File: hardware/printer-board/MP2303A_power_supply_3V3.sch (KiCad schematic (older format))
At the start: 10 parts, among them U12 MP2303A_ALT

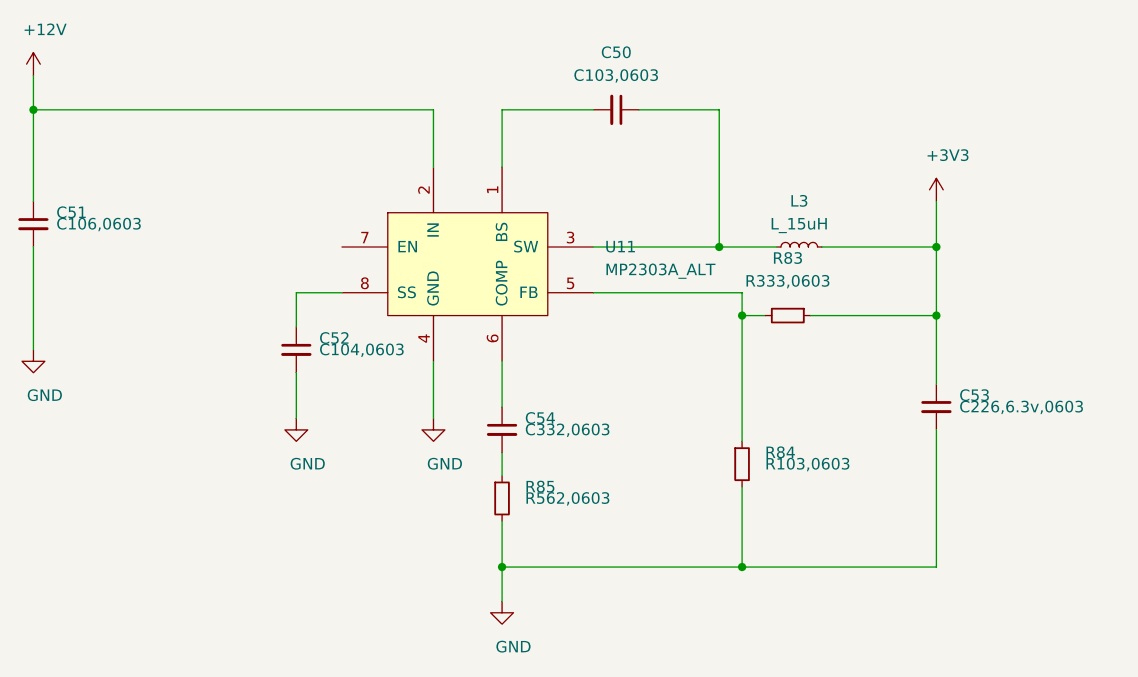
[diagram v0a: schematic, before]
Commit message: update to re-annotation,
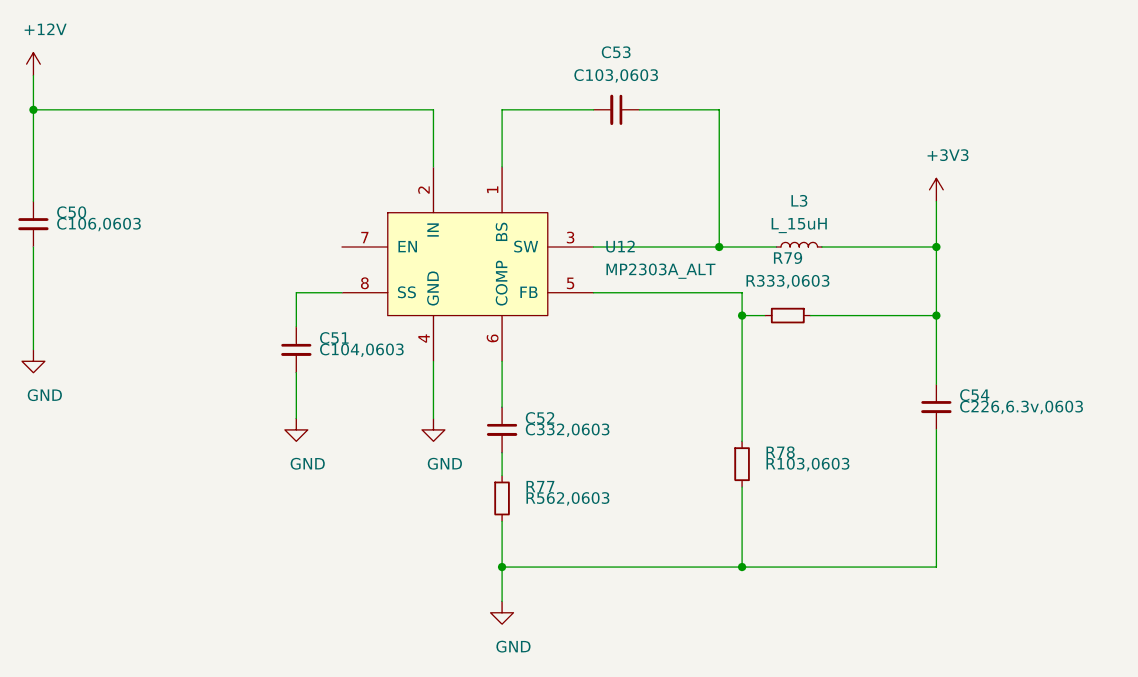
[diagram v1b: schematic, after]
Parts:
- U12: footprint Package_SO:SOIC-8_3.9x4.9mm_P1.27mm -> footprint-lib:SOIC-8_3.9x4.9mm_P1.27mm,thermal_via
- renumbered C54 to C52, C49 to C53, C53 to C54, L4 to L3, R91 to R77, R90 to R78, R89 to R79
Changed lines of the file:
@@
 $Descr A4 11693 8268
 encoding utf-8
-Sheet 34 29
+Sheet 29 29
 Title ""
 Date ""
@@
 $EndBitmap
 $Comp
-L taobao-components:MP2303A_ALT U12
+L taobao-components:MP2303A_ALT U?
 U 1 1 5CCACF42
 P 5000 3500
-AR Path="/5CC86276/5CCACF42" Ref="U12"  Part="1"
+AR Path="/5CC86276/5CCACF42" Ref="U?"  Part="1"
 AR Path="/5CCA7EF8/5CCACF42" Ref="U?"  Part="1"
 AR Path="/5CC29851/5CCA8098/5CCACF42" Ref="U?"  Part="1"
-AR Path="/5CCA8A04/5CCACF42" Ref="U11"  Part="1"
-F 0 "U11" H 5600 3550 50  0000 L CNN
+AR Path="/5CCA8A04/5CCACF42" Ref="U12"  Part="1"
+F 0 "U12" H 5600 3550 50  0000 L CNN
 F 1 "MP2303A_ALT" H 5600 3450 50  0000 L CNN
-F 2 "Package_SO:SOIC-8_3.9x4.9mm_P1.27mm" H 5000 3500 50  0001 C CNN
+F 2 "footprint-lib:SOIC-8_3.9x4.9mm_P1.27mm,thermal_via" H 5000 3500 50  0001 C CNN
 F 3 "" H 5000 3500 50  0001 C CNN
 	1    5000 3500
@@
 $EndComp
 $Comp
-L power:+12V #PWR0131
+L power:+12V #PWR?
 U 1 1 5CCACF43
 P 3100 2700
-AR Path="/5CC86276/5CCACF43" Ref="#PWR0131"  Part="1"
+AR Path="/5CC86276/5CCACF43" Ref="#PWR?"  Part="1"
 AR Path="/5CCA7EF8/5CCACF43" Ref="#PWR?"  Part="1"
 AR Path="/5CC29851/5CCA8098/5CCACF43" Ref="#PWR?"  Part="1"
-AR Path="/5CCA8A04/5CCACF43" Ref="#PWR0125"  Part="1"
-F 0 "#PWR0125" H 3100 2550 50  0001 C CNN
+AR Path="/5CCA8A04/5CCACF43" Ref="#PWR0209"  Part="1"
+F 0 "#PWR0209" H 3100 2550 50  0001 C CNN
 F 1 "+12V" H 3150 2900 50  0000 C CNN
 F 2 "" H 3100 2700 50  0001 C CNN
@@
 	3100 2700 3100 2850
 $Comp
-L power:GND #PWR0136
+L power:GND #PWR?
 U 1 1 5CCACF44
 P 3100 3900
-AR Path="/5CC86276/5CCACF44" Ref="#PWR0136"  Part="1"
+AR Path="/5CC86276/5CCACF44" Ref="#PWR?"  Part="1"
 AR Path="/5CCA7EF8/5CCACF44" Ref="#PWR?"  Part="1"
 AR Path="/5CC29851/5CCA8098/5CCACF44" Ref="#PWR?"  Part="1"
-AR Path="/5CCA8A04/5CCACF44" Ref="#PWR0131"  Part="1"
-F 0 "#PWR0131" H 3100 3650 50  0001 C CNN
+AR Path="/5CCA8A04/5CCACF44" Ref="#PWR0210"  Part="1"
+F 0 "#PWR0210" H 3100 3650 50  0001 C CNN
 F 1 "GND" H 3150 3700 50  0000 C CNN
 F 2 "" H 3100 3900 50  0001 C CNN
@@
 	3100 2850 3100 3250
 $Comp
-L taobao-c:C104,0603 C51
+L taobao-c:C104,0603 C?
 U 1 1 5CC8BF75
 P 4250 3900
-AR Path="/5CC86276/5CC8BF75" Ref="C51"  Part="1"
+AR Path="/5CC86276/5CC8BF75" Ref="C?"  Part="1"
 AR Path="/5CCA7EF8/5CC8BF75" Ref="C?"  Part="1"
 AR Path="/5CC29851/5CCA8098/5CC8BF75" Ref="C?"  Part="1"
-AR Path="/5CCA8A04/5CC8BF75" Ref="C52"  Part="1"
-F 0 "C52" H 4350 3950 50  0000 L CNN
+AR Path="/5CCA8A04/5CC8BF75" Ref="C51"  Part="1"
+F 0 "C51" H 4350 3950 50  0000 L CNN
 F 1 "C104,0603" H 4350 3900 50  0000 L CNN
 F 2 "Capacitor_SMD:C_0603_1608Metric_Pad1.05x0.95mm_HandSolder" H 4250 3900 50  0001 C CNN
@@
 	4250 3650 4450 3650
 $Comp
-L power:GND #PWR0141
+L power:GND #PWR?
 U 1 1 5CCACF46
 P 4250 4200
-AR Path="/5CC86276/5CCACF46" Ref="#PWR0141"  Part="1"
+AR Path="/5CC86276/5CCACF46" Ref="#PWR?"  Part="1"
 AR Path="/5CCA7EF8/5CCACF46" Ref="#PWR?"  Part="1"
 AR Path="/5CC29851/5CCA8098/5CCACF46" Ref="#PWR?"  Part="1"
-AR Path="/5CCA8A04/5CCACF46" Ref="#PWR0132"  Part="1"
-F 0 "#PWR0132" H 4250 3950 50  0001 C CNN
+AR Path="/5CCA8A04/5CCACF46" Ref="#PWR0211"  Part="1"
+F 0 "#PWR0211" H 4250 3950 50  0001 C CNN
 F 1 "GND" H 4300 4000 50  0000 C CNN
 F 2 "" H 4250 4200 50  0001 C CNN
@@
 	4250 4200 4250 4000
 $Comp
-L power:GND #PWR0142
+L power:GND #PWR?
 U 1 1 5CCACF47
 P 4850 4200
-AR Path="/5CC86276/5CCACF47" Ref="#PWR0142"  Part="1"
+AR Path="/5CC86276/5CCACF47" Ref="#PWR?"  Part="1"
 AR Path="/5CCA7EF8/5CCACF47" Ref="#PWR?"  Part="1"
 AR Path="/5CC29851/5CCA8098/5CCACF47" Ref="#PWR?"  Part="1"
-AR Path="/5CCA8A04/5CCACF47" Ref="#PWR0136"  Part="1"
-F 0 "#PWR0136" H 4850 3950 50  0001 C CNN
+AR Path="/5CCA8A04/5CCACF47" Ref="#PWR0212"  Part="1"
+F 0 "#PWR0212" H 4850 3950 50  0001 C CNN
 F 1 "GND" H 4900 4000 50  0000 C CNN
 F 2 "" H 4850 4200 50  0001 C CNN
@@
 	4850 4200 4850 3950
 $Comp
-L taobao-c:C103,0603 C49
+L taobao-c:C103,0603 C?
 U 1 1 5CCACF48
 P 5650 2850
-AR Path="/5CC86276/5CCACF48" Ref="C49"  Part="1"
+AR Path="/5CC86276/5CCACF48" Ref="C?"  Part="1"
 AR Path="/5CCA7EF8/5CCACF48" Ref="C?"  Part="1"
 AR Path="/5CC29851/5CCA8098/5CCACF48" Ref="C?"  Part="1"
-AR Path="/5CCA8A04/5CCACF48" Ref="C50"  Part="1"
-F 0 "C50" V 5400 2850 50  0000 C CNN
+AR Path="/5CCA8A04/5CCACF48" Ref="C53"  Part="1"
+F 0 "C53" V 5400 2850 50  0000 C CNN
 F 1 "C103,0603" V 5500 2850 50  0000 C CNN
 F 2 "Capacitor_SMD:C_0603_1608Metric_Pad1.05x0.95mm_HandSolder" H 5650 2850 50  0001 C CNN
@@
 	5150 2850 5150 3100
 $Comp
-L taobao-l:L_15uH L4
+L taobao-l:L_15uH L?
 U 1 1 5CCACF49
 P 6450 3450
-AR Path="/5CC86276/5CCACF49" Ref="L4"  Part="1"
+AR Path="/5CC86276/5CCACF49" Ref="L?"  Part="1"
 AR Path="/5CCA7EF8/5CCACF49" Ref="L?"  Part="1"
 AR Path="/5CC29851/5CCA8098/5CCACF49" Ref="L?"  Part="1"
@@
 	6100 3450 6350 3450
 $Comp
-L taobao-r:R562,0603 R91
+L taobao-r:R562,0603 R?
 U 1 1 5CCACF4A
 P 5150 4550
-AR Path="/5CC86276/5CCACF4A" Ref="R91"  Part="1"
+AR Path="/5CC86276/5CCACF4A" Ref="R?"  Part="1"
 AR Path="/5CCA7EF8/5CCACF4A" Ref="R?"  Part="1"
 AR Path="/5CC29851/5CCA8098/5CCACF4A" Ref="R?"  Part="1"
-AR Path="/5CCA8A04/5CCACF4A" Ref="R85"  Part="1"
-F 0 "R85" H 5250 4600 50  0000 L CNN
+AR Path="/5CCA8A04/5CCACF4A" Ref="R77"  Part="1"
+F 0 "R77" H 5250 4600 50  0000 L CNN
 F 1 "R562,0603" H 5250 4550 50  0000 L CNN
 F 2 "Resistor_SMD:R_0603_1608Metric_Pad1.05x0.95mm_HandSolder" H 5150 4550 50  0001 C CNN
@@
 $EndComp
 $Comp
-L power:GND #PWR0143
+L power:GND #PWR?
 U 1 1 5CCACF4B
 P 5150 5000
-AR Path="/5CC86276/5CCACF4B" Ref="#PWR0143"  Part="1"
+AR Path="/5CC86276/5CCACF4B" Ref="#PWR?"  Part="1"
 AR Path="/5CCA7EF8/5CCACF4B" Ref="#PWR?"  Part="1"
 AR Path="/5CC29851/5CCA8098/5CCACF4B" Ref="#PWR?"  Part="1"
-AR Path="/5CCA8A04/5CCACF4B" Ref="#PWR0141"  Part="1"
-F 0 "#PWR0141" H 5150 4750 50  0001 C CNN
+AR Path="/5CCA8A04/5CCACF4B" Ref="#PWR0213"  Part="1"
+F 0 "#PWR0213" H 5150 4750 50  0001 C CNN
 F 1 "GND" H 5200 4800 50  0000 C CNN
 F 2 "" H 5150 5000 50  0001 C CNN
@@
 $EndComp
 $Comp
-L taobao-c:C332,0603 C54
+L taobao-c:C332,0603 C?
 U 1 1 5CCACF4C
 P 5150 4250
-AR Path="/5CC86276/5CCACF4C" Ref="C54"  Part="1"
+AR Path="/5CC86276/5CCACF4C" Ref="C?"  Part="1"
 AR Path="/5CCA7EF8/5CCACF4C" Ref="C?"  Part="1"
 AR Path="/5CC29851/5CCA8098/5CCACF4C" Ref="C?"  Part="1"
-AR Path="/5CCA8A04/5CCACF4C" Ref="C54"  Part="1"
-F 0 "C54" H 5250 4300 50  0000 L CNN
+AR Path="/5CCA8A04/5CCACF4C" Ref="C52"  Part="1"
+F 0 "C52" H 5250 4300 50  0000 L CNN
 F 1 "C332,0603" H 5250 4250 50  0000 L CNN
 F 2 "Capacitor_SMD:C_0603_1608Metric_Pad1.05x0.95mm_HandSolder" H 5150 4250 50  0001 C CNN
@@
 	5150 4650 5150 4850
 $Comp
-L taobao-r:R103,0603 R90
+L taobao-r:R103,0603 R?
 U 1 1 5CC8CDDD
 P 6200 4400
-AR Path="/5CC86276/5CC8CDDD" Ref="R90"  Part="1"
+AR Path="/5CC86276/5CC8CDDD" Ref="R?"  Part="1"
 AR Path="/5CCA7EF8/5CC8CDDD" Ref="R?"  Part="1"
 AR Path="/5CC29851/5CCA8098/5CC8CDDD" Ref="R?"  Part="1"
-AR Path="/5CCA8A04/5CC8CDDD" Ref="R84"  Part="1"
-F 0 "R84" H 6300 4450 50  0000 L CNN
+AR Path="/5CCA8A04/5CC8CDDD" Ref="R78"  Part="1"
+F 0 "R78" H 6300 4450 50  0000 L CNN
 F 1 "R103,0603" H 6300 4400 50  0000 L CNN
 F 2 "Resistor_SMD:R_0603_1608Metric_Pad1.05x0.95mm_HandSolder" H 6200 4400 50  0001 C CNN
@@
 $EndComp
 $Comp
-L taobao-r:R333,0603 R89
+L taobao-r:R333,0603 R?
 U 1 1 5CC8CF8B
 P 6400 3750
-AR Path="/5CC86276/5CC8CF8B" Ref="R89"  Part="1"
+AR Path="/5CC86276/5CC8CF8B" Ref="R?"  Part="1"
 AR Path="/5CCA7EF8/5CC8CF8B" Ref="R?"  Part="1"
 AR Path="/5CC29851/5CCA8098/5CC8CF8B" Ref="R?"  Part="1"
-AR Path="/5CCA8A04/5CC8CF8B" Ref="R83"  Part="1"
-F 0 "R83" V 6150 3750 50  0000 C CNN
+AR Path="/5CCA8A04/5CC8CF8B" Ref="R79"  Part="1"
+F 0 "R79" V 6150 3750 50  0000 C CNN
 F 1 "R333,0603" V 6250 3750 50  0000 C CNN
 F 2 "Resistor_SMD:R_0603_1608Metric_Pad1.05x0.95mm_HandSolder" H 6400 3750 50  0001 C CNN
@@
 	6200 4850 7050 4850
 $Comp
-L taobao-c:C226,6.3v,0603 C53
+L taobao-c:C226,6.3v,0603 C?
 U 1 1 5CCACF4F
 P 7050 4150
-AR Path="/5CC86276/5CCACF4F" Ref="C53"  Part="1"
+AR Path="/5CC86276/5CCACF4F" Ref="C?"  Part="1"
 AR Path="/5CCA7EF8/5CCACF4F" Ref="C?"  Part="1"
 AR Path="/5CC29851/5CCA8098/5CCACF4F" Ref="C?"  Part="1"
-AR Path="/5CCA8A04/5CCACF4F" Ref="C53"  Part="1"
-F 0 "C53" H 7150 4200 50  0000 L CNN
+AR Path="/5CCA8A04/5CCACF4F" Ref="C54"  Part="1"
+F 0 "C54" H 7150 4200 50  0000 L CNN
 F 1 "C226,6.3v,0603" H 7150 4150 50  0000 L CNN
 F 2 "Capacitor_SMD:C_0603_1608Metric_Pad1.05x0.95mm_HandSolder" H 7050 4150 50  0001 C CNN
@@
 $EndComp
 $Comp
-L taobao-c:C106,0603 C50
+L taobao-c:C106,0603 C?
 U 1 1 5CC95CF5
 P 3100 3350
-AR Path="/5CC86276/5CC95CF5" Ref="C50"  Part="1"
+AR Path="/5CC86276/5CC95CF5" Ref="C?"  Part="1"
 AR Path="/5CCA7EF8/5CC95CF5" Ref="C?"  Part="1"
 AR Path="/5CC29851/5CCA8098/5CC95CF5" Ref="C?"  Part="1"
-AR Path="/5CCA8A04/5CC95CF5" Ref="C51"  Part="1"
-F 0 "C51" H 3200 3400 50  0000 L CNN
+AR Path="/5CCA8A04/5CC95CF5" Ref="C50"  Part="1"
+F 0 "C50" H 3200 3400 50  0000 L CNN
 F 1 "C106,0603" H 3200 3350 50  0000 L CNN
 F 2 "Capacitor_SMD:C_0603_1608Metric_Pad1.05x0.95mm_HandSolder" H 3100 3350 50  0001 C CNN
@@
 $EndComp
 $Comp
-L power:+3V3 #PWR0130
+L power:+3V3 #PWR0214
 U 1 1 5CCA8FAD
 P 7050 3250
-F 0 "#PWR0130" H 7050 3100 50  0001 C CNN
+F 0 "#PWR0214" H 7050 3100 50  0001 C CNN
 F 1 "+3V3" H 7100 3450 50  0000 C CNN
 F 2 "" H 7050 3250 50  0001 C CNN
